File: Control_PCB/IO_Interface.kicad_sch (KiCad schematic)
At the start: 95 parts, among them Q10 BCX56, Q11 BCX56, Q12 BC846, Q13 BC846, Q14 BCX56, Q4 BCX56, Q6 BC846, Q7 BCX56, Q8 BC846, Q9 PUMH11, U6 TCAN1043xDxQ1, U7 TLIN2021

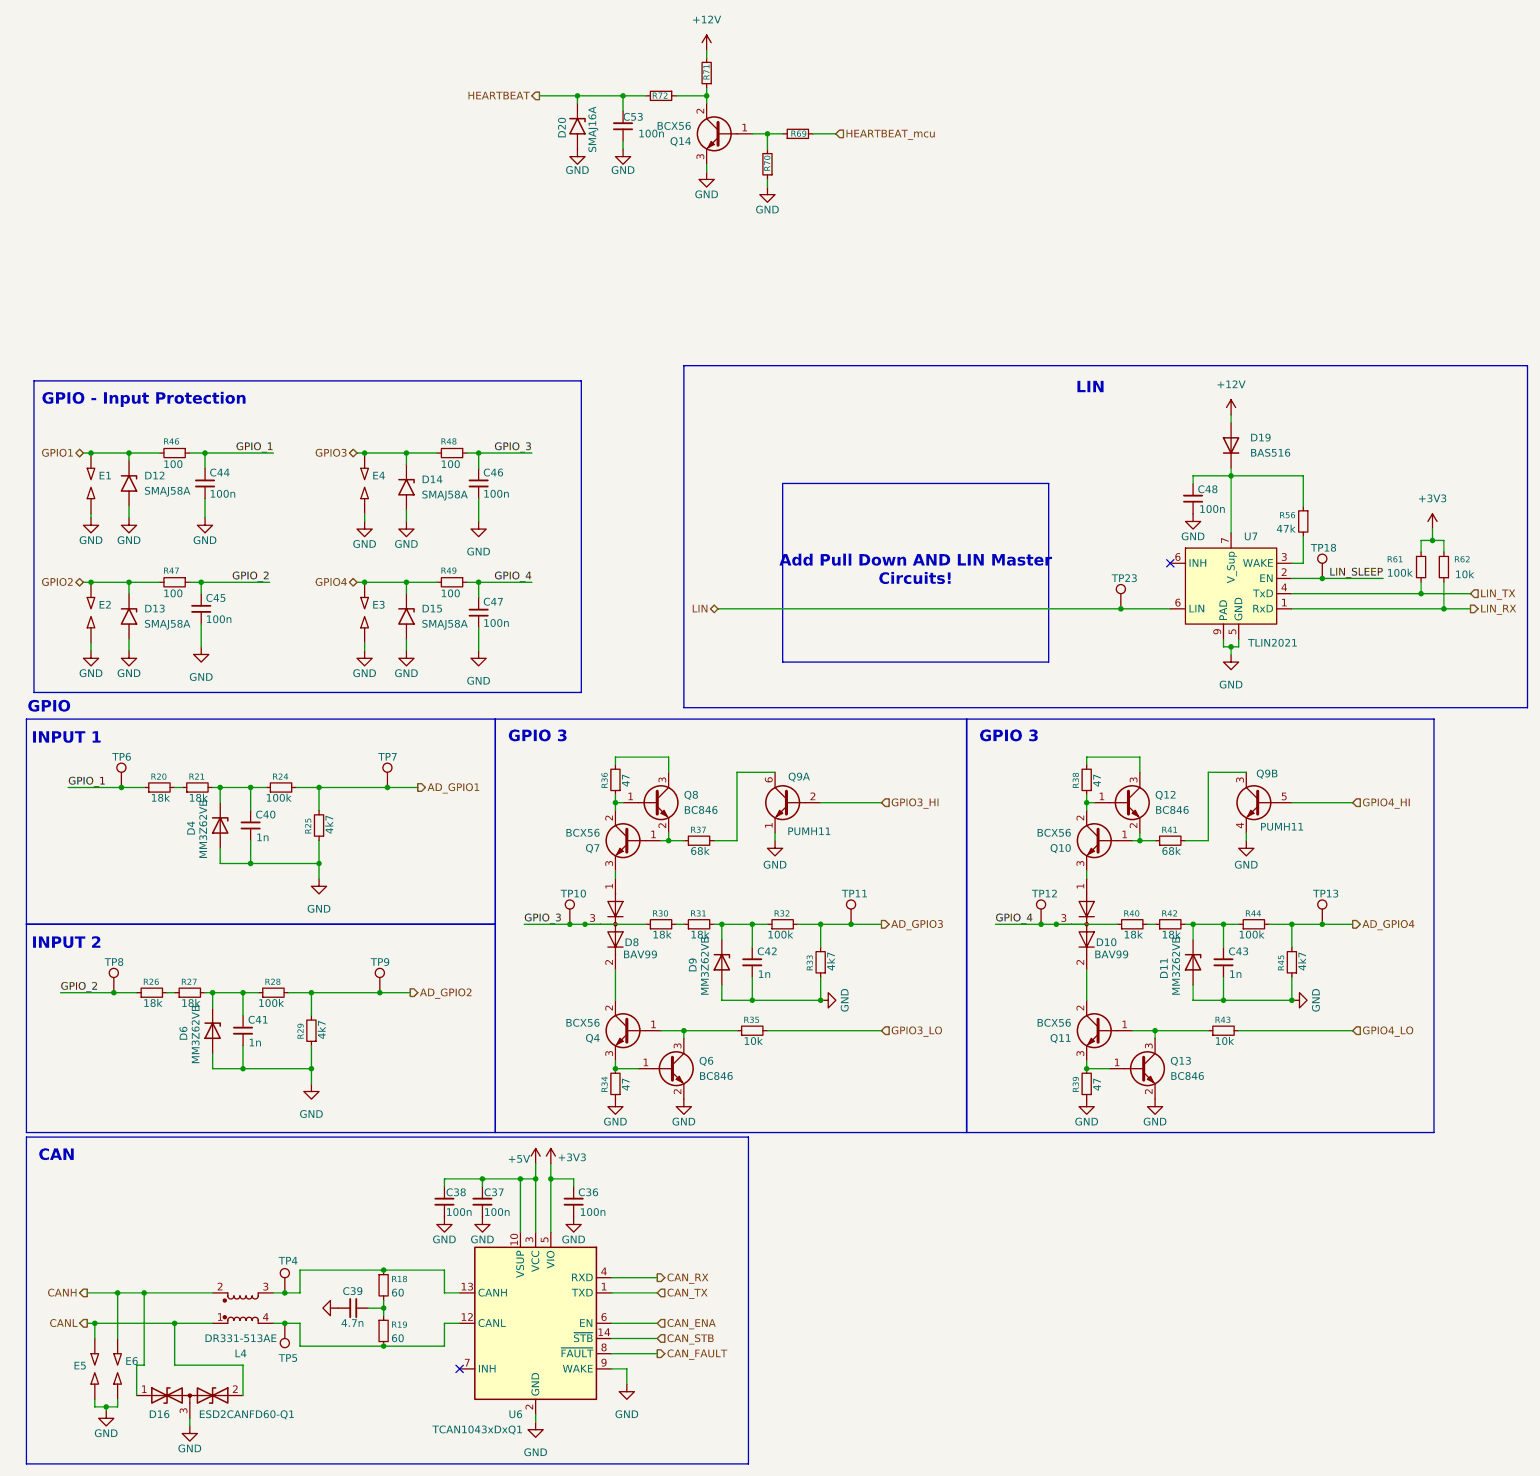
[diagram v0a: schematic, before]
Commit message: 15-10-2026
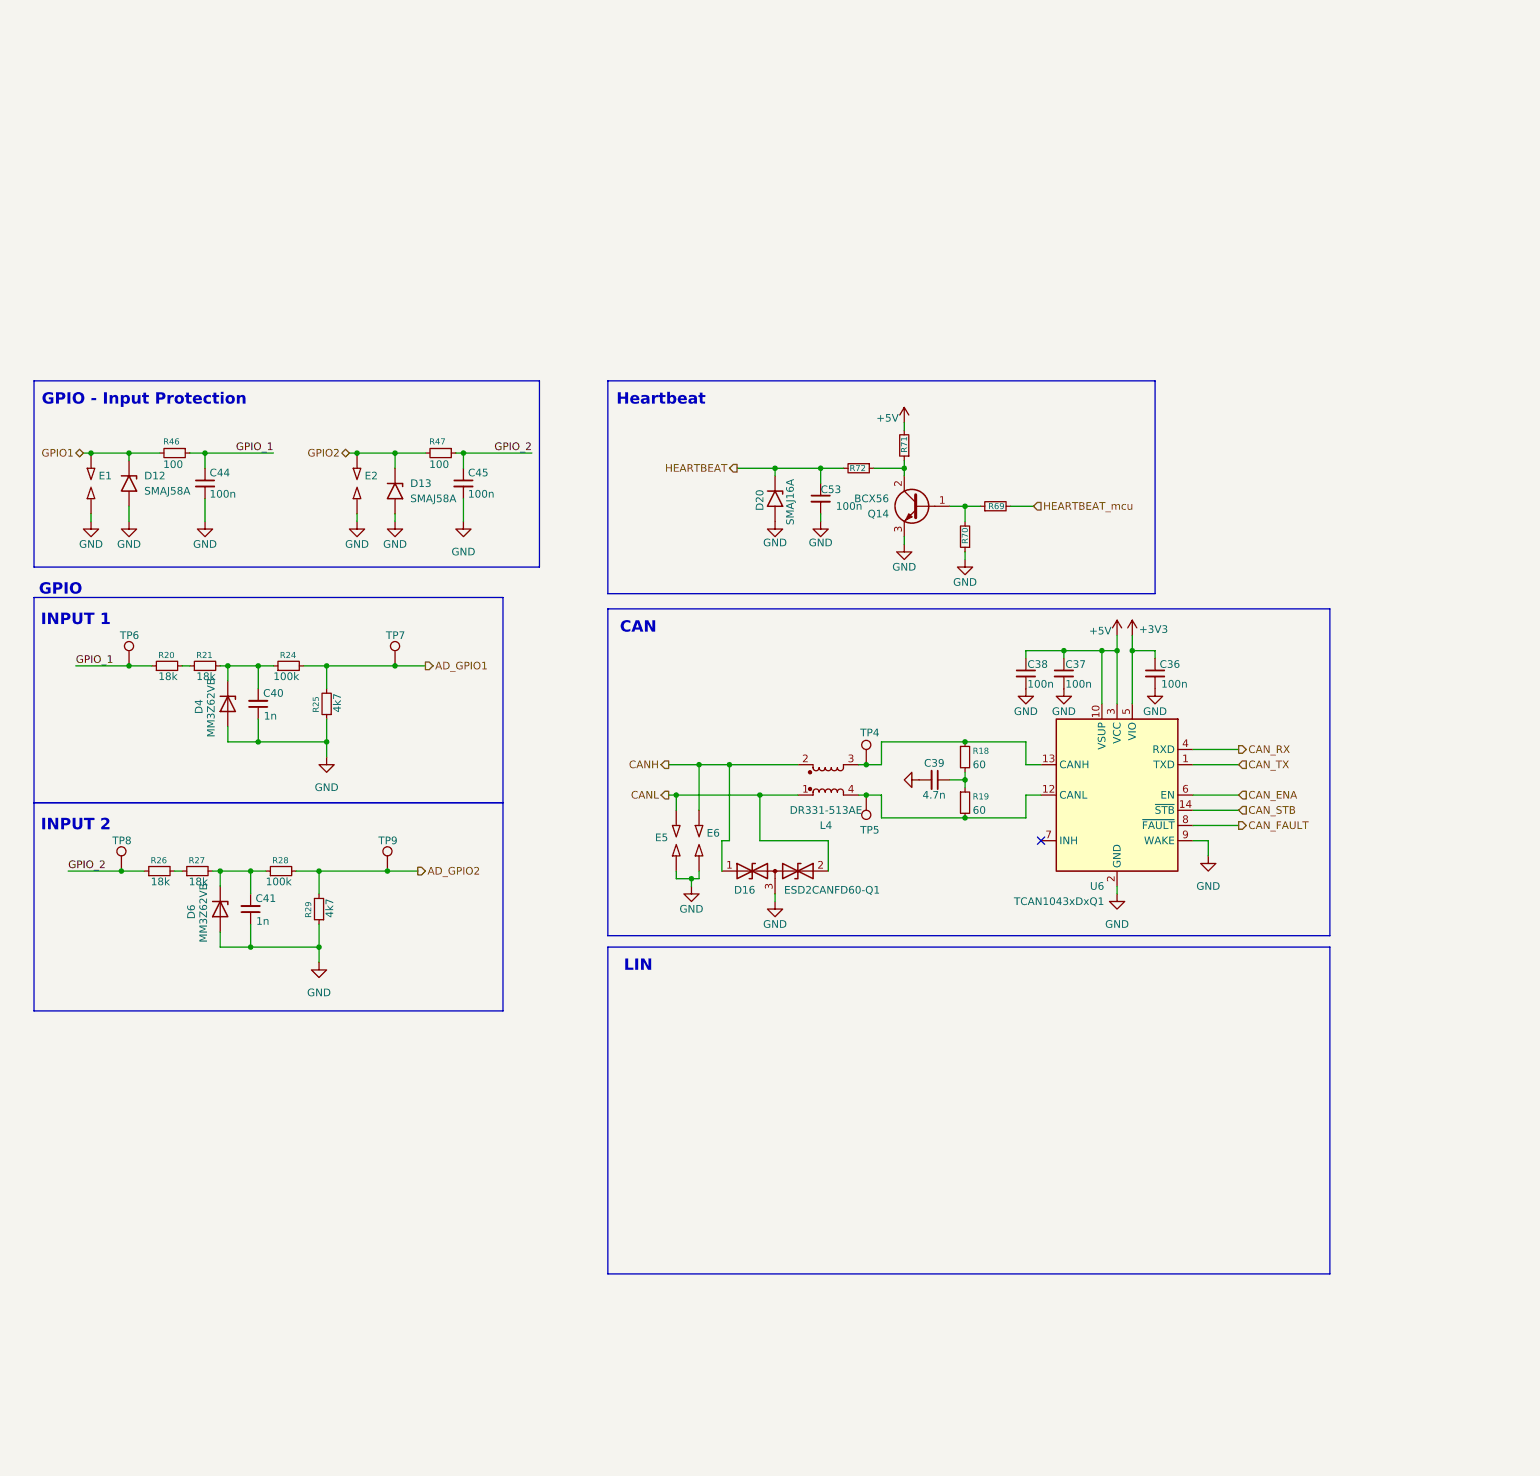
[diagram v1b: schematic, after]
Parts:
- removed C42, C43: 1n, Capacitor_SMD:C_0603_1608Metric, symbol Device:C_Small
- removed C46, C47, C48: 100n, Capacitor_SMD:C_0603_1608Metric, symbol Device:C_Small
- removed D10, D8: BAV99, Package_TO_SOT_SMD:SOT-23, symbol Diode:BAV99
- removed D11, D9: MM3Z62VB, Diode_SMD:D_SOD-323F, symbol Diode:MM3Zxx
- removed D14, D15: SMAJ58A, Diode_SMD:D_SMA, symbol Diode:SMAJ58A
- removed D19: BAS516, Diode_SMD:D_SOD-523, symbol Diode:BAS516
- removed E3, E4: SparkGap, Control_PCB:Sparkgap_2021-09-02, symbol Device:SparkGap
- removed Q10, Q11, Q4, Q7: BCX56, Package_TO_SOT_SMD:SOT-89-3, symbol Transistor_BJT:BCX56
- removed Q12, Q13, Q6, Q8: BC846, Package_TO_SOT_SMD:SOT-23, symbol Transistor_BJT:BC846
- removed Q9: PUMH11, Package_TO_SOT_SMD:SOT-363_SC-70-6, symbol Transistor_BJT:PUMX1
- removed R30, R31, R40, R42: 18k, Resistor_SMD:R_0603_1608Metric, symbol Device:R_Small
- removed R32, R44, R61: 100k, Resistor_SMD:R_0603_1608Metric, symbol Device:R_Small
- removed R33, R45: 4k7, Resistor_SMD:R_0603_1608Metric, symbol Device:R_Small
- removed R34, R36, R38, R39: 47, Resistor_SMD:R_0603_1608Metric, symbol Device:R_Small
- removed R35, R43, R62: 10k, Resistor_SMD:R_0603_1608Metric, symbol Device:R_Small
- removed R37, R41: 68k, Resistor_SMD:R_0603_1608Metric, symbol Device:R_Small
- removed R48, R49: 100, Resistor_SMD:R_1206_3216Metric, symbol Device:R_Small
- removed R56: 47k, Resistor_SMD:R_0603_1608Metric, symbol Device:R_Small
- removed TP10, TP11, TP12, TP13, TP18, TP23: TestPoint, TestPoint:TestPoint_Pad_D1.5mm, symbol Connector:TestPoint
- removed U7: TLIN2021, Package_SO:SOIC-8_5.3x5.3mm_P1.27mm, symbol Control_PCB:TLIN2021
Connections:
- net +12V is gone; now on net +5V: R71.2
- no-connect marks 2 -> 1
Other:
- note added: "Heartbeat"
- note removed: "Add Pull Down AND LIN Master Circuits!"
- note removed: "GPIO 3"
- moved on the sheet: C36, C37, C38, C39, C40, C41, C45, C53, D13, D16, D20, D4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
